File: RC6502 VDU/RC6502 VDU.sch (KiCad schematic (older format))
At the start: 39 parts, among them J1 RC6502_Backplane, J2 VDU_BASE, J3 VIDEO, J4 Hole, J5 Hole, J6 Hole, J7 Hole, J8 RCA_PLUG, Q1 PN2222A, Q2 PN2222A, U1 MC6847, U10 74HCT00, U2 HM62256BLP-7, U3 74LS244, U4 74LS244, U5 74LS245, U6 74LS374, U7 74HCT138, U8 74HCT04, U9 74HCT00, X1 3.579545 MHz

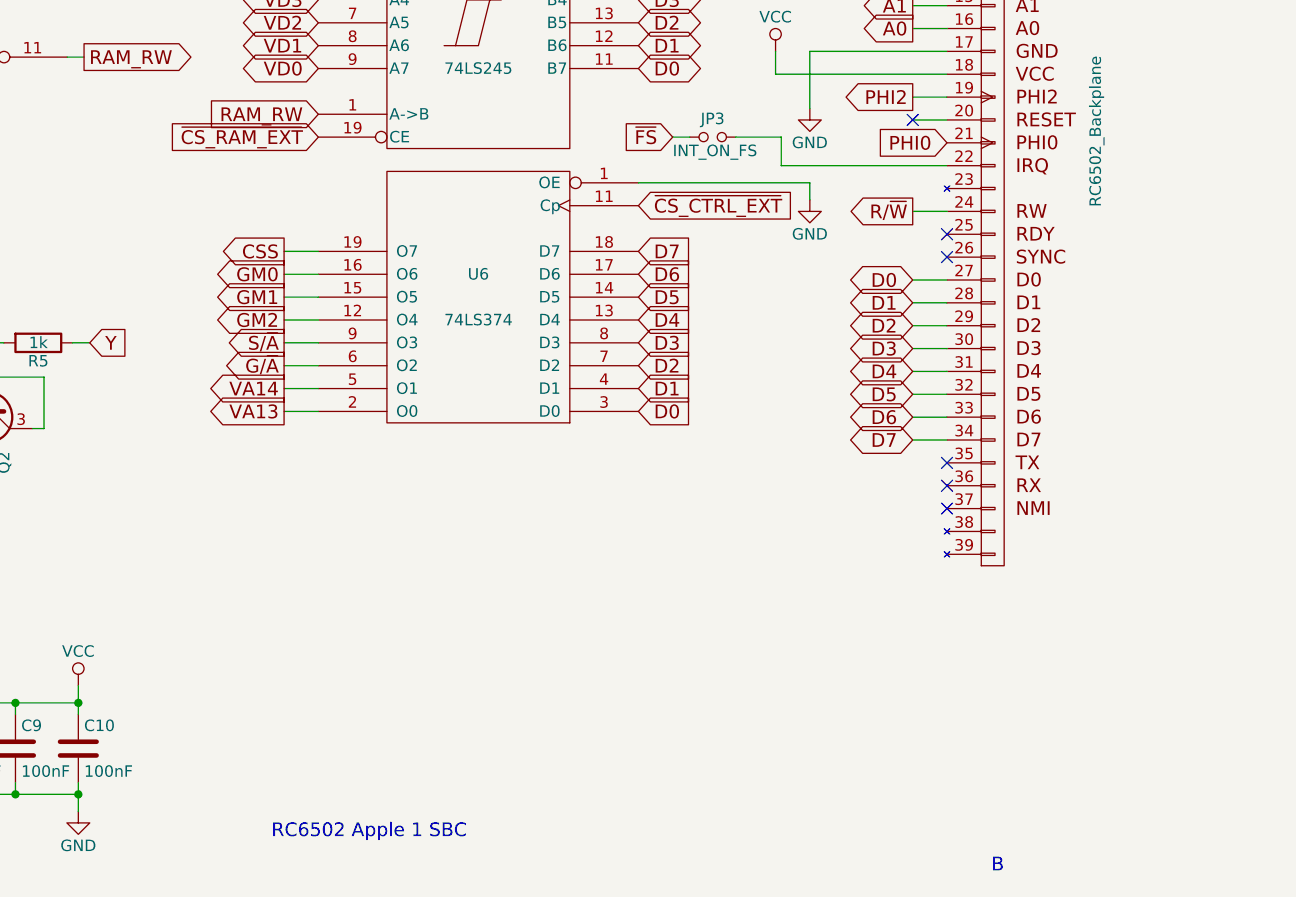
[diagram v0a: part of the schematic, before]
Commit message: Added description
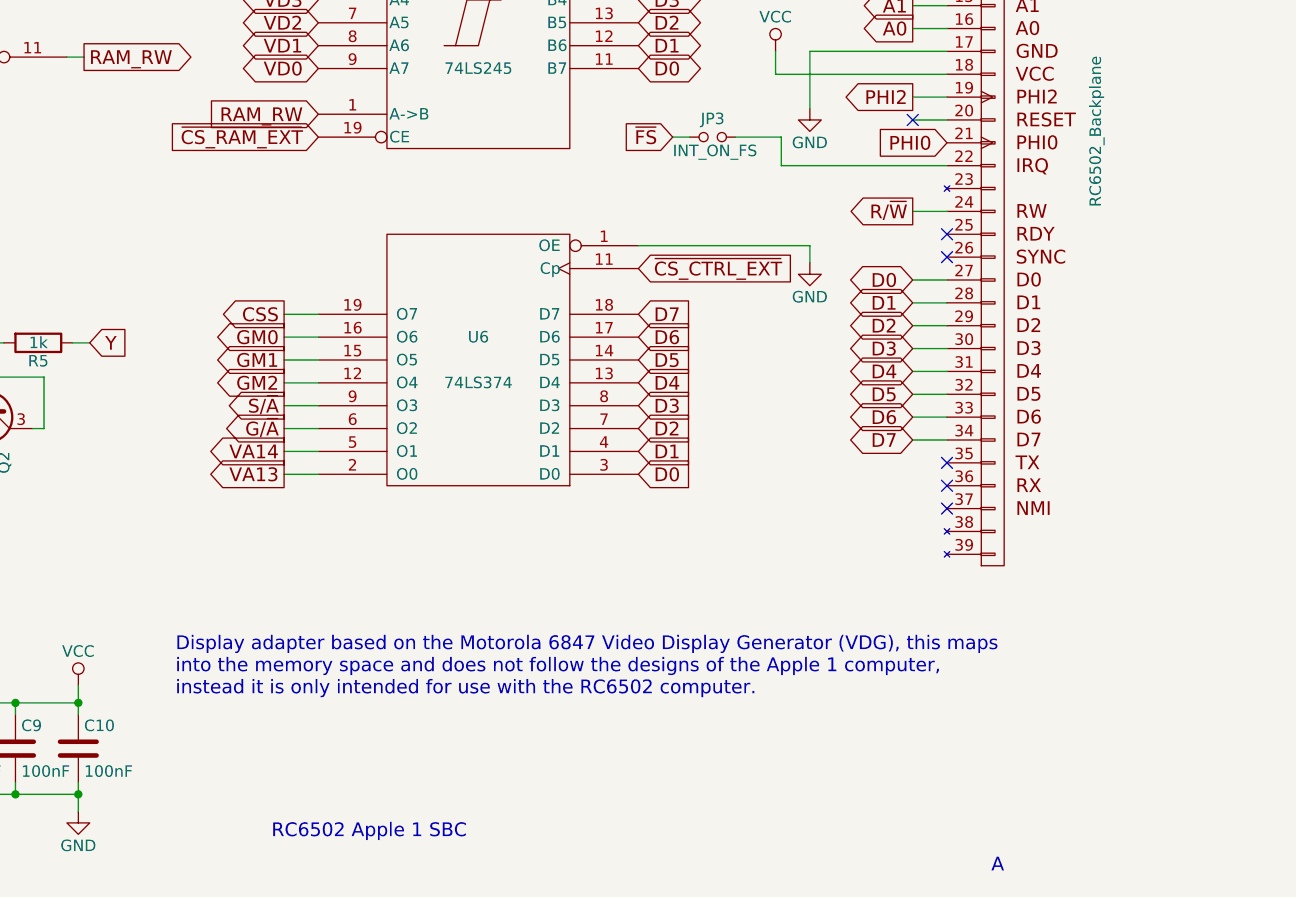
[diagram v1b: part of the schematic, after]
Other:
- note added: "A"
- note added: "Display adapter based on the Motorola 6847 Video Display Generator (VDG), this maps\ninto the memory space and does not follow the designs of the Apple 1 computer,\ninstead it is only intended for use with the RC6502 computer."
- note removed: "B"
- moved on the sheet: U6
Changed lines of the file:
@@
 RC6502 Apple 1 SBC
 Text Notes 10650 7650 2    60   ~ 0
-B
+A
 $Comp
 L 74LS138 U7
@@
 L 74LS374 U6
 U 1 1 5C049977
-P 8350 5125
-F 0 "U6" H 8350 5025 50  0000 C CNN
-F 1 "74LS374" H 8350 5225 50  0000 C CNN
-F 2 "" H 8350 5125 50  0001 C CNN
-F 3 "" H 8350 5125 50  0001 C CNN
-	1    8350 5125
+P 8350 5400
+F 0 "U6" H 8350 5300 50  0000 C CNN
+F 1 "74LS374" H 8350 5500 50  0000 C CNN
+F 2 "" H 8350 5400 50  0001 C CNN
+F 3 "" H 8350 5400 50  0001 C CNN
+	1    8350 5400
 	-1   0    0    1
 $EndComp
-Text GLabel 9050 4925 2    60   Input ~ 0
+Text GLabel 9050 5200 2    60   Input ~ 0
 D7
-Text GLabel 9050 5025 2    60   Input ~ 0
+Text GLabel 9050 5300 2    60   Input ~ 0
 D6
-Text GLabel 9050 5125 2    60   Input ~ 0
+Text GLabel 9050 5400 2    60   Input ~ 0
 D5
-Text GLabel 9050 5225 2    60   Input ~ 0
+Text GLabel 9050 5500 2    60   Input ~ 0
 D4
-Text GLabel 9050 5325 2    60   Input ~ 0
+Text GLabel 9050 5600 2    60   Input ~ 0
 D3
-Text GLabel 9050 5425 2    60   Input ~ 0
+Text GLabel 9050 5700 2    60   Input ~ 0
 D2
-Text GLabel 9050 5525 2    60   Input ~ 0
+Text GLabel 9050 5800 2    60   Input ~ 0
 D1
-Text GLabel 9050 5625 2    60   Input ~ 0
+Text GLabel 9050 5900 2    60   Input ~ 0
 D0
 $Comp
@@
 L GND #PWR08
 U 1 1 5C04E709
-P 9800 4700
-F 0 "#PWR08" H 9800 4450 50  0001 C CNN
-F 1 "GND" H 9800 4550 50  0000 C CNN
-F 2 "" H 9800 4700 50  0001 C CNN
-F 3 "" H 9800 4700 50  0001 C CNN
-	1    9800 4700
-	1    0    0    -1
-$EndComp
-Wire Wire Line
-	9050 4625 9800 4625
+P 9800 4975
+F 0 "#PWR08" H 9800 4725 50  0001 C CNN
+F 1 "GND" H 9800 4825 50  0000 C CNN
+F 2 "" H 9800 4975 50  0001 C CNN
+F 3 "" H 9800 4975 50  0001 C CNN
+	1    9800 4975
+	1    0    0    -1
+$EndComp
+Wire Wire Line
+	9050 4900 9800 4900
 Text GLabel 7650 3425 0    60   BiDi ~ 0
 VD7
@@
 Text GLabel 925  6850 0    60   Input ~ 0
 VA8
-Text GLabel 7500 5525 0    60   Output ~ 0
+Text GLabel 7500 5800 0    60   Output ~ 0
 VA14
-Text GLabel 7500 5625 0    60   Output ~ 0
+Text GLabel 7500 5900 0    60   Output ~ 0
 VA13
 Text GLabel 925  7450 0    60   Input ~ 0
@@
 NoConn ~ 6250 2950
 Wire Wire Line
-	7500 5525 7650 5525
-Wire Wire Line
-	7500 5625 7650 5625
+	7500 5800 7650 5800
+Wire Wire Line
+	7500 5900 7650 5900
 Text GLabel 10400 4450 0    60   Input ~ 0
 PHI0
@@
 Text GLabel 6250 2050 2    60   Input ~ 0
 G/~A
-Text GLabel 7500 5425 0    60   Output ~ 0
+Text GLabel 7500 5700 0    60   Output ~ 0
 G/~A
 Text GLabel 6250 2150 2    60   Input ~ 0
 S/~A
-Text GLabel 7500 5325 0    60   Output ~ 0
+Text GLabel 7500 5600 0    60   Output ~ 0
 S/~A
 Text GLabel 6250 2350 2    60   Input ~ 0
@@
 Text GLabel 6250 2650 2    60   Input ~ 0
 CSS
-Text GLabel 7500 4925 0    60   Output ~ 0
+Text GLabel 7500 5200 0    60   Output ~ 0
 CSS
-Text GLabel 7500 5025 0    60   Output ~ 0
+Text GLabel 7500 5300 0    60   Output ~ 0
 GM0
-Text GLabel 7500 5125 0    60   Output ~ 0
+Text GLabel 7500 5400 0    60   Output ~ 0
 GM1
-Text GLabel 7500 5225 0    60   Output ~ 0
+Text GLabel 7500 5500 0    60   Output ~ 0
 GM2
 Wire Wire Line
-	7500 4925 7650 4925
-Wire Wire Line
-	7650 5025 7500 5025
-Wire Wire Line
-	7500 5125 7650 5125
-Wire Wire Line
-	7650 5225 7500 5225
-Wire Wire Line
-	7500 5325 7650 5325
-Wire Wire Line
-	7650 5425 7500 5425
+	7500 5200 7650 5200
+Wire Wire Line
+	7650 5300 7500 5300
+Wire Wire Line
+	7500 5400 7650 5400
+Wire Wire Line
+	7650 5500 7500 5500
+Wire Wire Line
+	7500 5600 7650 5600
+Wire Wire Line
+	7650 5700 7500 5700
 $Comp
 L GND #PWR010
@@
 Wire Wire Line
 	3500 925  3575 925
-Text GLabel 9050 4725 2    60   Input ~ 0
+Text GLabel 9050 5000 2    60   Input ~ 0
 ~CS_CTRL_EXT
 Text GLabel 9200 725  2    60   Input ~ 0
@@
 ~VDU_WRITE
 Wire Wire Line
-	9800 4625 9800 4700
+	9800 4900 9800 4975
 Wire Wire Line
 	2025 5050 2100 5050
@@
 Wire Wire Line
 	4900 5575 4900 5650
+Text Notes 7025 6875 0    60   ~ 0
+Display adapter based on the Motorola 6847 Video Display Generator (VDG), this maps\ninto the memory space and does not follow the designs of the Apple 1 computer,\ninstead it is only intended for use with the RC6502 computer.
 $EndSCHEMATC
